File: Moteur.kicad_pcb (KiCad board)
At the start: 2 copper layers, 0 parts

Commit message: Couche PCB Définie
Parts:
- added C10: 10n, _0603, F.Cu at (76.2, 72.4)
- added C11, C12: 10pF, _0603, F.Cu at (0.00, 0.00)
- added C13, C6, C7, C9: 100n, _0603, F.Cu at (0.00, 0.00)
- added C14, C16: 47nF, SM1206, F.Cu at (0.00, 0.00)
- added C15: 47nF, SM1206, F.Cu at (48.3, 69.8)
- added R11: 100k, SM0805, F.Cu at (59.7, 52.1)
- added R8: 100k, SM0805, F.Cu at (34.3, 29.2)
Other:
- copper layers 2 -> 4
- net class Default: clearance 0.254 -> 0.204; trace_width 0.254 -> 0.204; via_dia 0.889 -> 0.8; via_drill 0.635 -> 0.3
- rule trace_clearance: 0.254 -> 0.204
- rule trace_min: 0.254 -> 0.204
- rule via_min_drill: 0.508 -> 0.3
- rule via_min_size: 0.889 -> 0.8

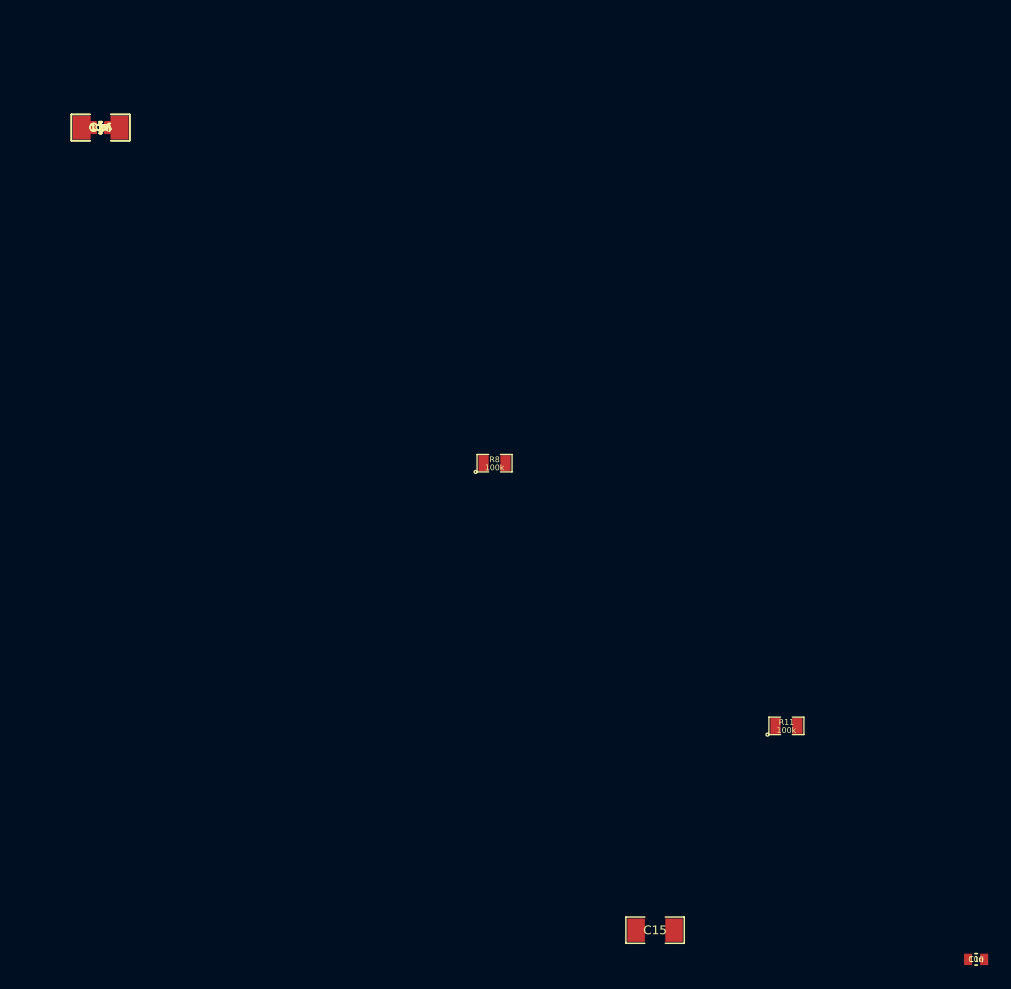
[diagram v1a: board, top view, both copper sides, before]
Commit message: footprints
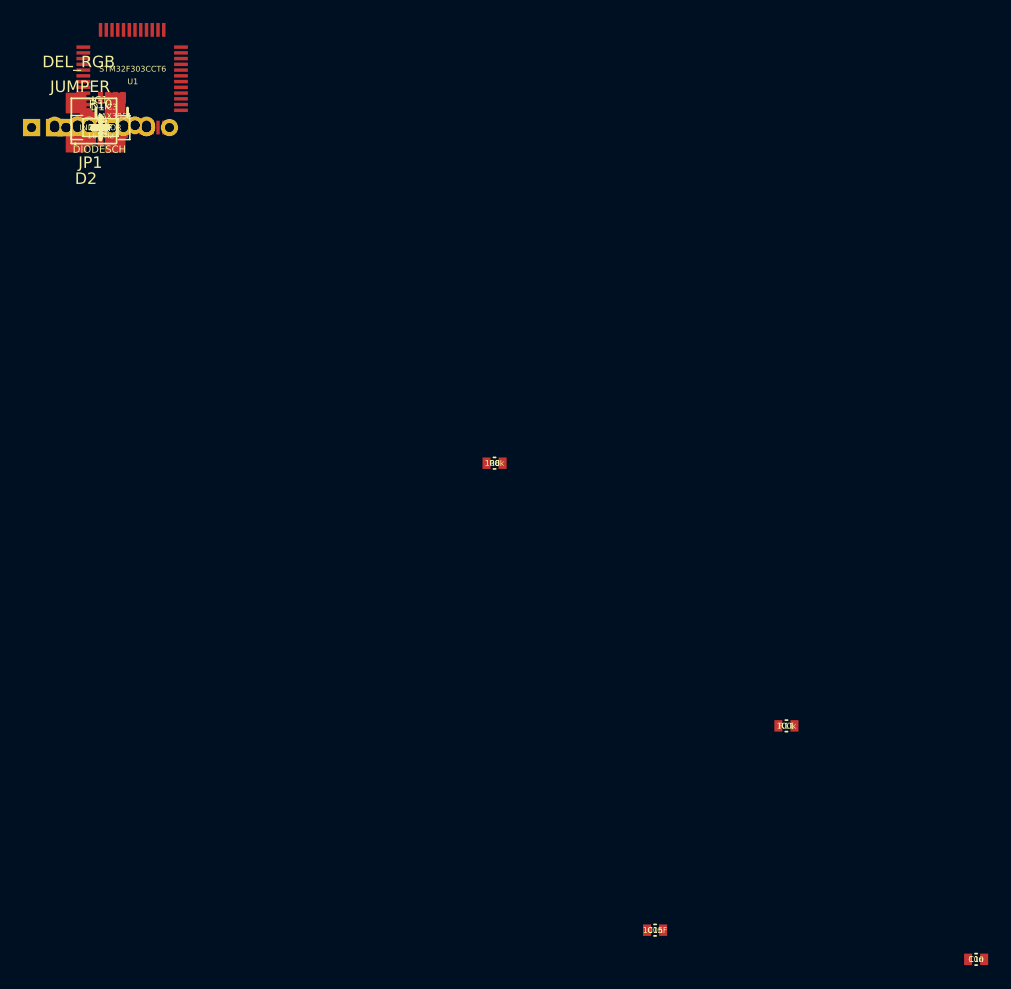
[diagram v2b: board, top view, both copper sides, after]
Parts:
- added C1, C5: 100n, _0603, F.Cu at (0.00, 0.00)
- added C17, C8: 1uF, _0603, F.Cu at (0.00, 0.00)
- added C18: C, _0603, F.Cu at (0.00, 0.00)
- added C2: 100nF, _0603, F.Cu at (0.00, 0.00)
- added C3: 4.7uF, _0603, F.Cu at (0.00, 0.00)
- added C4: 470n, _0603, F.Cu at (0.00, 0.00)
- added D1: DIODESCH, CVRA-SOD80C, F.Cu at (0.00, 0.00)
- added D2: DEL_RGB, LedRGB, F.Cu at (0.00, 0.00)
- added IC1: TPS71501, CVRA-SOT23-5, F.Cu at (0.00, 0.00)
- added IC3: MAX3051, _SOT23-8, F.Cu at (0.00, 0.00)
- added JP1: JUMPER, Jumer, F.Cu at (0.00, 0.00)
- added L1: INDUCTOR, _0603, F.Cu at (0.00, 0.00)
- added P1: Bus2, _Pin2mm_4z, F.Cu at (0.00, 0.00)
- added P2: MotorEnc, _Pin2mm_5z, F.Cu at (0.00, 0.00)
- added P3: Bus1, _Pin2mm_4z, F.Cu at (0.00, 0.00)
- added P4: Motor, _Pin2mm_2, F.Cu at (0.00, 0.00)
- added P5: DBG, _Pin2mm_7z, F.Cu at (0.00, 0.00)
- added P6: PWR, _Pin2mm_2, F.Cu at (0.00, 0.00)
- added P7: GPIO, _Pin2mm_5z, F.Cu at (0.00, 0.00)
- added R1: 5.6M, _0603, F.Cu at (0.00, 0.00)
- added R10: 0.01R, CVRA-1206-1, F.Cu at (0.00, 0.00)
- added R12, R13: R, _0603, F.Cu at (0.00, 0.00)
- added R2: 910k, _0603, F.Cu at (0.00, 0.00)
- added R3: 0R, _0603, F.Cu at (0.00, 0.00)
- added R4: 22, _0603, F.Cu at (0.00, 0.00)
- added R5: 47, _0603, F.Cu at (0.00, 0.00)
- added R6: 39, _0603, F.Cu at (0.00, 0.00)
- added R7: 120, _0603, F.Cu at (0.00, 0.00)
- added R9: 330, _0603, F.Cu at (0.00, 0.00)
- added U1: STM32F303CCT6, _LQFP48, F.Cu at (0.00, 0.00)
- added X1: 16MHz, _TSX-3225-SMD-XTAL, F.Cu at (0.00, 0.00)
- C14, C16: footprint SM1206 -> _0603
- C15: value 47nF -> 100nF; footprint SM1206 -> _0603
- R11, R8: footprint SM0805 -> _0603
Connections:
- C10 pad 1: N-000002 -> +3.3V_A
